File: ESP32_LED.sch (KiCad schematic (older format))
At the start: 45 parts, among them J1 5077CR-16SMC2-BK-TR, J2 Conn_01x15, J3 Conn_01x15, J4 Servo0, J5 Servo1, J6 Servo2, J7 Servo3, J8 Iris, Q1 2SC4081, Q2 2SC4081, SW1 MODE, SW2 RESET, U1 CP2104-F03-GM, U2 ESP-WROOM-32, U3 TC2117

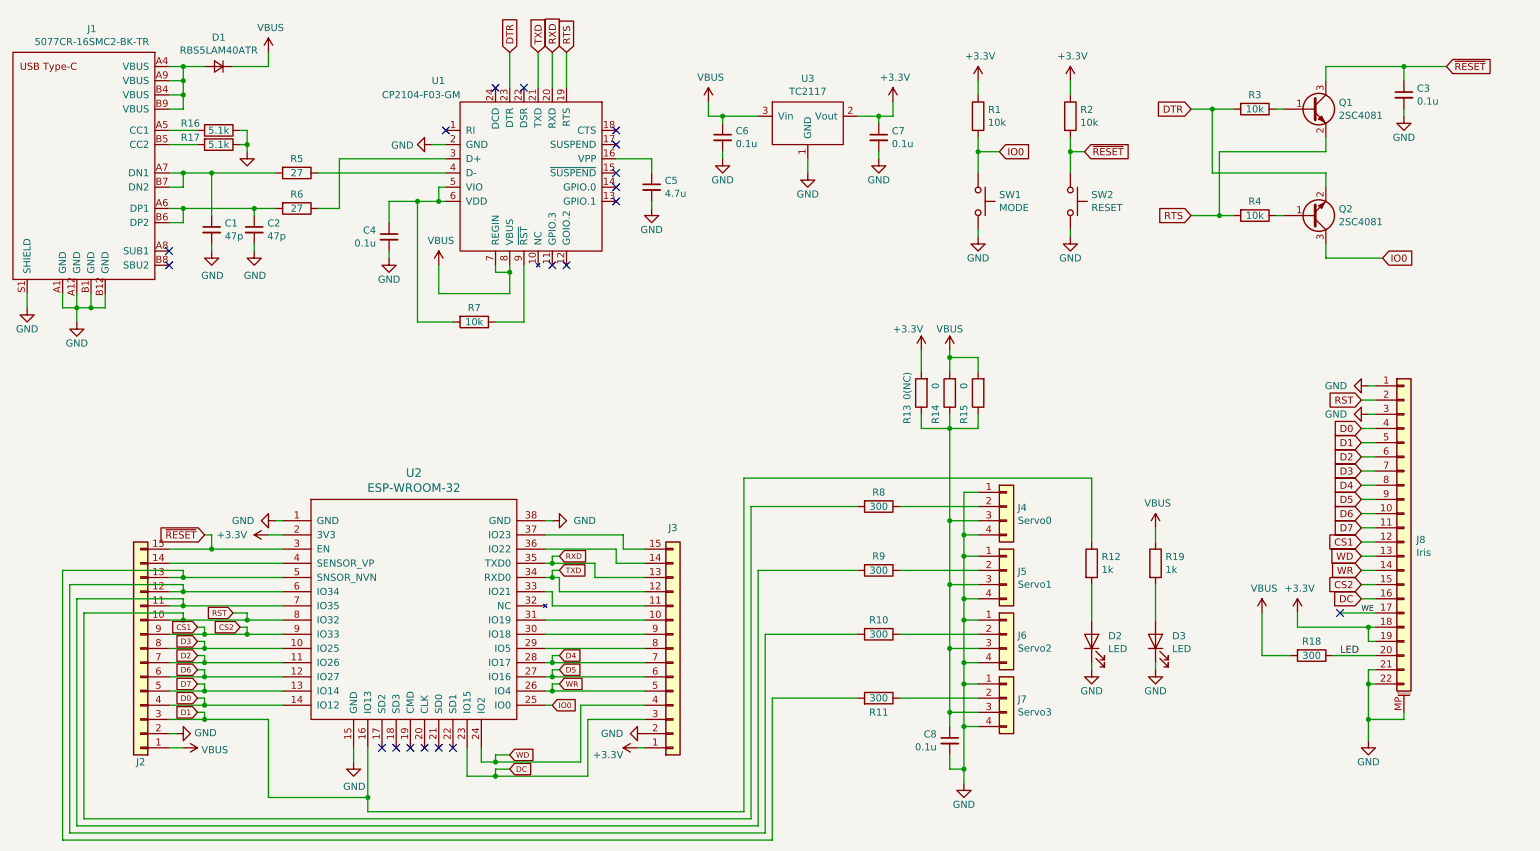
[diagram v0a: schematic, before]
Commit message: rev1.1
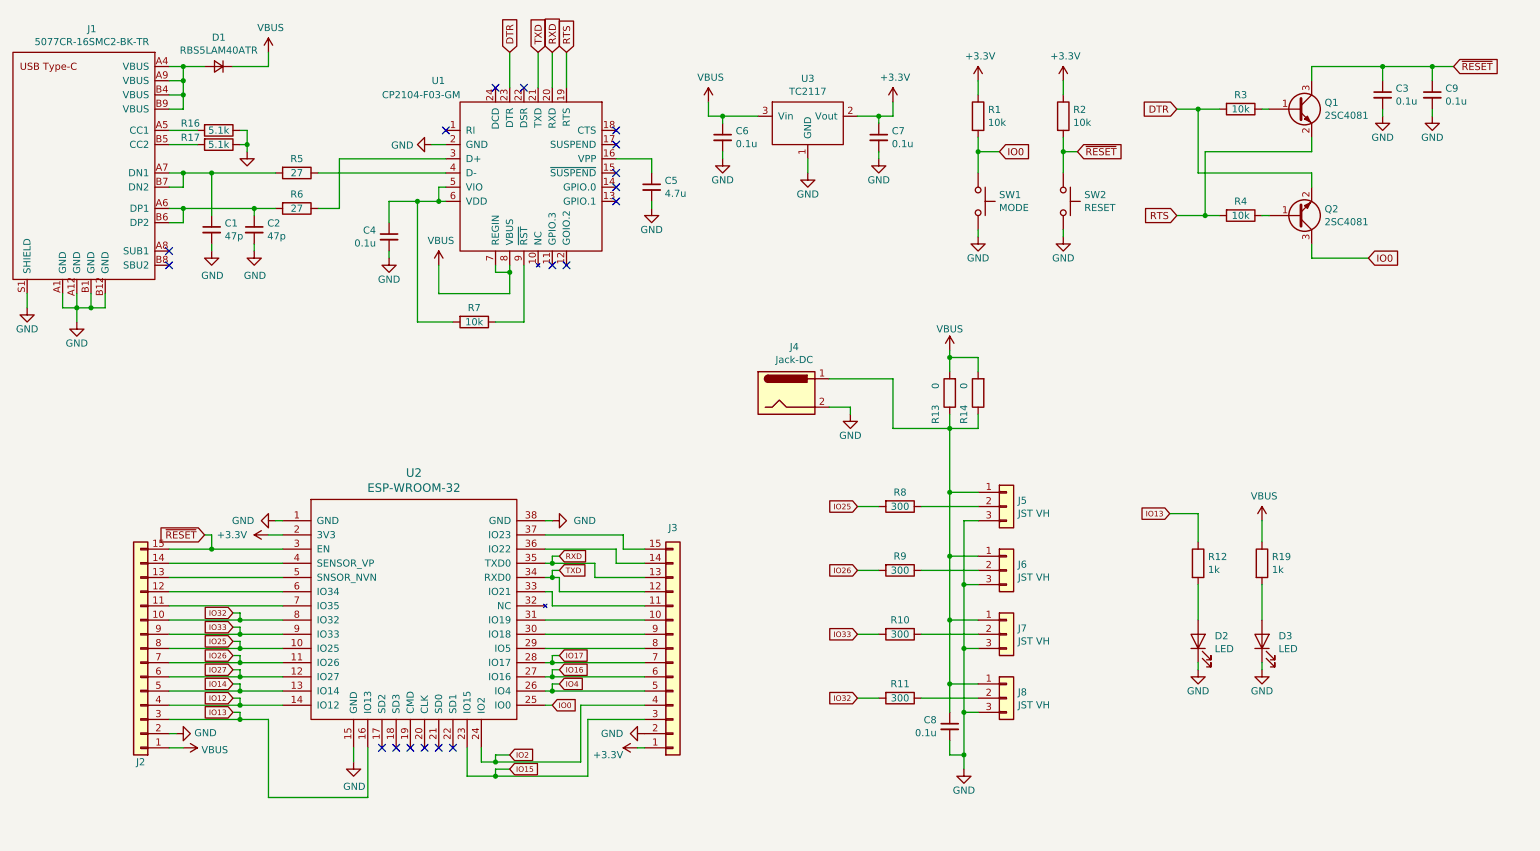
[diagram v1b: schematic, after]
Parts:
- removed J4: Servo0, Connector_PinHeader_2.54mm:PinHeader_1x04_P2.54mm_Vertical, symbol Connector_Generic:Conn_01x04
- removed J5: Servo1, Connector_PinHeader_2.54mm:PinHeader_1x04_P2.54mm_Vertical, symbol Connector_Generic:Conn_01x04
- removed J6: Servo2, Connector_PinHeader_2.54mm:PinHeader_1x04_P2.54mm_Vertical, symbol Connector_Generic:Conn_01x04
- removed J7: Servo3, Connector_PinHeader_2.54mm:PinHeader_1x04_P2.54mm_Vertical, symbol Connector_Generic:Conn_01x04
- removed J8: Iris, Connector_FFC-FPC:Hirose_FH12-22S-0.5SH_1x22-1MP_P0.50mm_Horizontal, symbol Connector_Generic_MountingPin:Conn_01x22_MountingPin
- removed R15: 0, Resistor_SMD:R_0805_2012Metric, symbol Device:R
- removed R18: 300, Resistor_SMD:R_0402_1005Metric, symbol Device:R
- added C9: 0.1u, Capacitor_SMD:C_0402_1005Metric, symbol Device:C_Small
- added J4: Jack-DC, akizuki:2DC-G213-D42, symbol Connector:Jack-DC
- added J5, J6, J7, J8: JST VH, Connector_JST:JST_VH_B3P-VH-B_1x03_P3.96mm_Vertical, symbol Connector_Generic:Conn_01x03
- R13: value 0(NC) -> 0
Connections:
- net +3V3: no longer R13.2
- net GND: now also C9.2, J4.2, J5.3 (Pin_3), J6.3 (Pin_3), J7.3 (Pin_3), J8.3 (Pin_3)
- net VBUS: now also R13.2
- net ~RESET: now also C9.1
- net at J2.13 (Pin_13), U2.5 (SNSOR_NVN): no longer R11.2
- net at J2.12 (Pin_12), U2.6 (IO34): no longer R10.2
- net at J2.11 (Pin_11), U2.7 (IO35): no longer R9.2
- net at R8.1: now also J5.2 (Pin_2)
- net at C8.1, R13.1, R14.1: now also J4.1, J5.1 (Pin_1), J6.1 (Pin_1), J7.1 (Pin_1), J8.1 (Pin_1)
- net at R9.1: now also J6.2 (Pin_2)
- net at R10.1: now also J7.2 (Pin_2)
- net at R11.1: now also J8.2 (Pin_2)
- net CS1 renamed IO33
- net IO33: now also R10.2
- net D0 renamed IO12
- net D1 renamed IO13
- net D2 renamed IO26
- net IO26: now also R9.2
- net D3 renamed IO25
- net IO25: now also R8.2
- net D4 renamed IO17
- net D5 renamed IO16
- net D6 renamed IO27
- net D7 renamed IO14
- net DC renamed IO15
- net RST renamed IO32
- net IO32: now also R11.2; no longer R8.2
- net WD renamed IO2
- net WR renamed IO4
- no-connect marks 19 -> 18
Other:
- moved on the sheet: C3, C8, D2, D3, Q1, Q2, R10, R12, R14, R19, R2, R3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
